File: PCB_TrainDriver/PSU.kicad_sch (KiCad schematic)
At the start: 20 parts, among them U8 TPSM863257RDXR, U9 LDL1117S33R

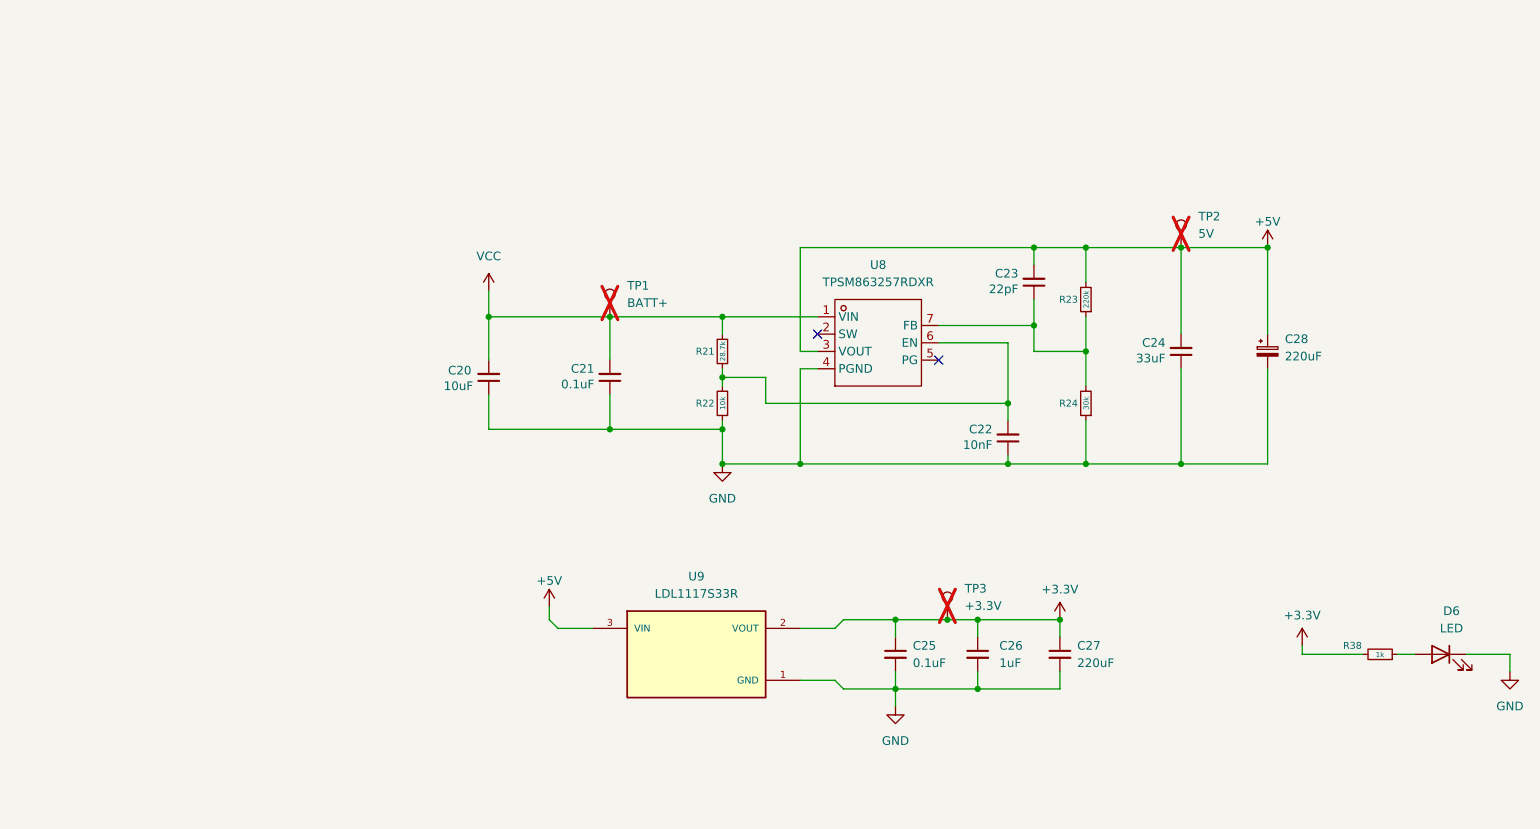
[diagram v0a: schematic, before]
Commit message: Finished sch
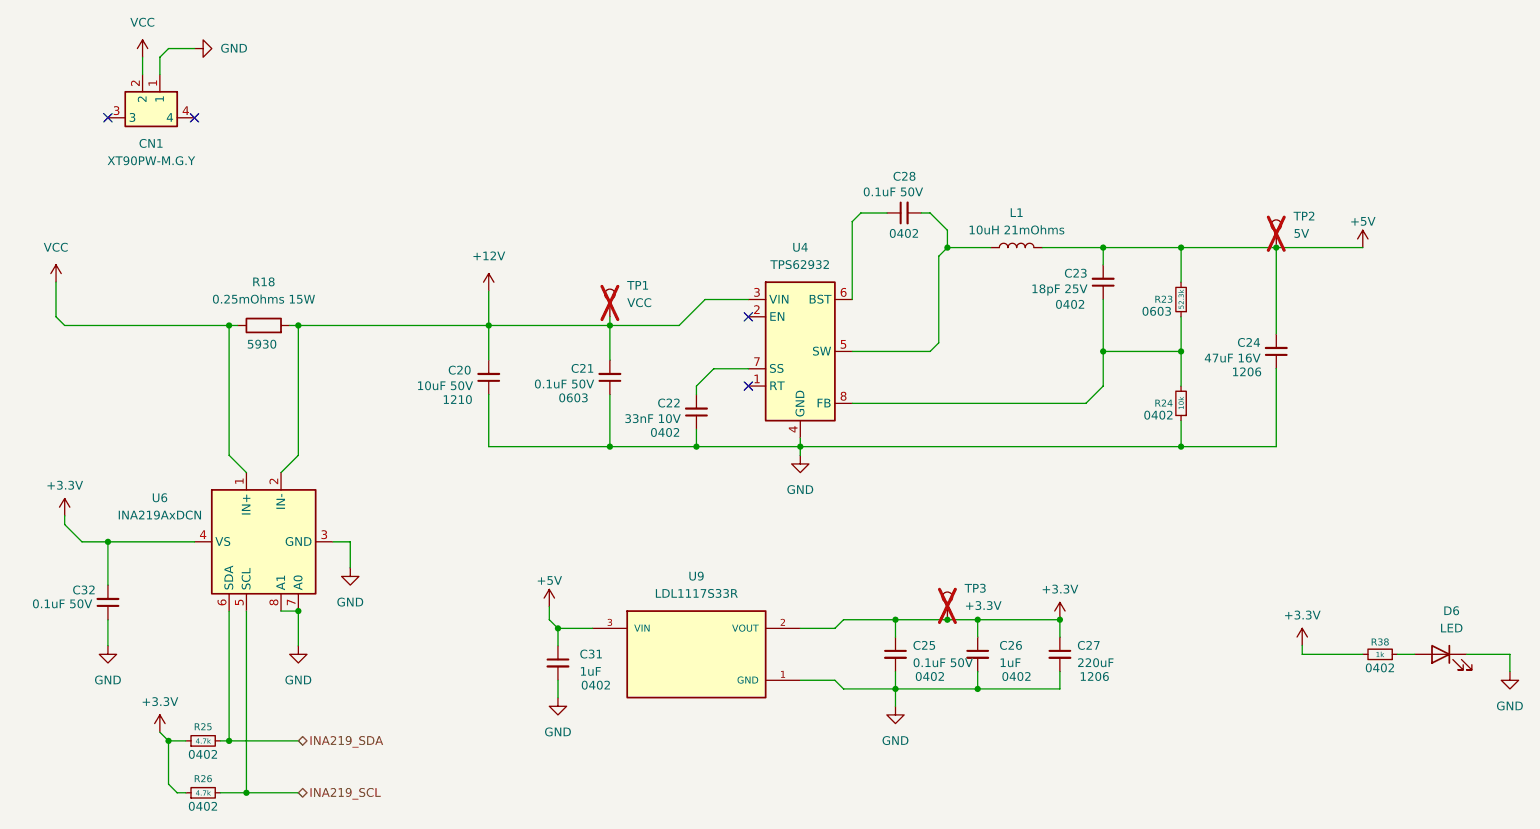
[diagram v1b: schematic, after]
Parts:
- removed C28: 220uF, Capacitor_SMD:CP_Elec_6.3x5.4, symbol Device:C_Polarized_Small
- removed R21: 28.7k, Resistor_SMD:R_0402_1005Metric, symbol Device:R_Small
- removed R22: 10k, Resistor_SMD:R_0402_1005Metric, symbol Device:R_Small
- removed U8: TPSM863257RDXR, SamacSys_Parts:QFN-7_L4.0-W3.3_TPSM863257RDXR, symbol SamacSys_Parts:TPSM863257RDXR
- added C28, C32: 0.1uF 50V, Capacitor_SMD:C_0402_1005Metric, symbol Device:C_Small
- added C31: 1uF, Capacitor_SMD:C_0402_1005Metric, symbol Device:C_Small
- added CN1: XT90PW-M.G.Y, Sharing_Footprint:CONN-TH_XT90PW-M.G.Y, symbol Sharing_Symbol:XT90PW-M.G.Y
- added L1: 10uH 21mOhms, Inductor_SMD:L_12x12mm_H4.5mm, symbol Device:L
- added R18: 0.25mOhms 15W, Sharing_Footprint:R5930, symbol Device:R
- added R25, R26: 4.7k, Resistor_SMD:R_0402_1005Metric, symbol Device:R_Small
- added U4: TPS62932, Package_TO_SOT_SMD:SOT-583-8, symbol Regulator_Switching:TPS62932
- added U6: INA219AxDCN, Package_TO_SOT_SMD:SOT-23-8, symbol Sensor_Energy:INA219AxDCN
- C20: value 10uF -> 10uF 50V; footprint Capacitor_SMD:C_0402_1005Metric -> Capacitor_SMD:C_1206_3216Metric; JLCPCB Part # (none) -> C13585; LCSC Part # C77000 -> (none); Package (none) -> 1210
- C21: value 0.1uF -> 0.1uF 50V; footprint Capacitor_SMD:C_0402_1005Metric -> Capacitor_SMD:C_0603_1608Metric; JLCPCB Part # (none) -> C14663; LCSC Part # C71687 -> (none); Package (none) -> 0603
- C22: value 10nF -> 33nF 10V; JLCPCB Part # (none) -> C527022; LCSC Part # C541371 -> (none); Package (none) -> 0402
- C23: value 22pF -> 18pF 25V; JLCPCB Part # (none) -> C526984; LCSC Part # C1555 -> (none); Package (none) -> 0402
- C24: value 33uF -> 47uF 16V; footprint Capacitor_SMD:C_0402_1005Metric -> Capacitor_SMD:C_1206_3216Metric; JLCPCB Part # (none) -> C7472975; LCSC Part # C1160 -> (none); Package (none) -> 1206
- C25: value 0.1uF -> 0.1uF 50V; JLCPCB Part # (none) -> C307331; LCSC Part # C71687 -> (none); LCSC Part# C1525 -> (none); Package (none) -> 0402
- C26: JLCPCB Part # (none) -> C52923; LCSC Part # C14445 -> (none); LCSC Part# C29266 -> (none); Package (none) -> 0402
- C27: JLCPCB Part # (none) -> C412252; LCSC Part # C412252 -> (none); LCSC Part# C412252 -> (none); Package (none) -> 1206
- D6: footprint LED_SMD:LED_0402_1005Metric -> LED_SMD:LED_0603_1608Metric; JLCPCB Part # (none) -> C2286; LCSC Part # C71911 -> (none)
- R23: value 220k -> 52.3k; footprint Resistor_SMD:R_0402_1005Metric -> Resistor_SMD:R_0603_1608Metric; JLCPCB Part # (none) -> C23198; LCSC Part # C25767 -> (none); Package (none) -> 0603
- R24: value 30k -> 10k; JLCPCB Part # (none) -> C25744; LCSC Part # C25553 -> (none); Package (none) -> 0402
- R38: JLCPCB Part # (none) -> C11702; LCSC Part # C106235 -> (none); Package (none) -> 0402
- TP1: value BATT+ -> VCC
- U9: JLCPCB Part # (none) -> C18906017; LCSC Part # C435835 -> (none); LCSC Part# C435835 -> (none)
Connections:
- net +3.3V: now also C32.2, R25.1, R26.1, U6.4 (VS)
- net +5V: now also C31.1, L1.2
- net GND: now also C31.2, C32.1, CN1.1, U4.4 (GND), U6.3 (GND), U6.7 (A0), U6.8 (A1)
- net VCC: now also CN1.2, R18.1, U6.1 (IN+); no longer C20.2, C21.2, TP1.1
- net at C22.2: now also U4.7 (SS)
- net at C23.1, R23.1, R24.2: now also U4.8 (FB)
- new net: C28.2, L1.1, U4.5 (SW)
- new net: C28.1, U4.6 (BST)
- new net +12V: C20.2, C21.2, R18.2, TP1.1, U4.3 (VIN), U6.2 (IN-)
- new net INA219_SCL: R26.2, U6.5 (SCL)
- new net INA219_SDA: R25.2, U6.6 (SDA)
- no-connect marks 2 -> 4
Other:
- moved on the sheet: C22, C23, C24, R23, R24, TP2

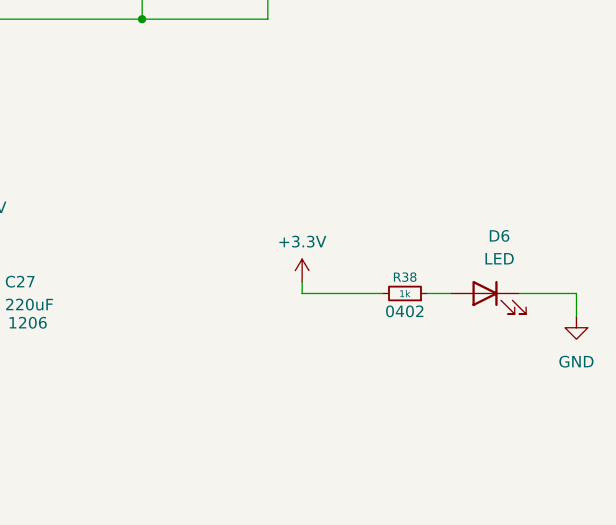
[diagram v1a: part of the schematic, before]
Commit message: PCB Almost Finished
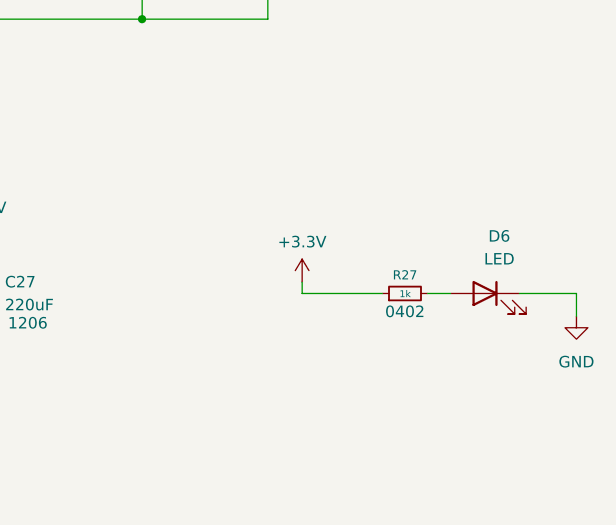
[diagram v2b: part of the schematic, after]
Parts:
- removed R38: 1k, Resistor_SMD:R_0402_1005Metric, symbol Device:R_Small
- added R27: 1k, Resistor_SMD:R_0402_1005Metric, symbol Device:R_Small
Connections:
- net +3.3V: now also R27.1
- net at D6.2 (A): now also R27.2
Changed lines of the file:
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@@
-	)
-	(symbol
-		(lib_id "Device:R_Small")
-		(at 218.44 142.24 270)
-		(mirror x)
-		(unit 1)
-		(body_style 1)
-		(exclude_from_sim no)
-		(in_bom yes)
-		(on_board no)
-		(in_pos_files yes)
-		(dnp no)
-		(property "Reference" "R38"
-			(at 218.44 140.462 90)
-			(show_name no)
-			(do_not_autoplace no)
-			(effects
-				(font
-					(size 1.016 1.016)
-				)
-			)
-		)
-		(property "Value" "1k"
-			(at 218.421 142.2933 90)
-			(show_name no)
-			(do_not_autoplace no)
-			(effects
-				(font
-					(size 0.762 0.762)
-				)
-			)
-		)
-		(property "Footprint" "Resistor_SMD:R_0402_1005Metric"
-			(at 218.44 142.24 0)
-			(hide yes)
-			(show_name no)
-			(do_not_autoplace no)
-			(effects
-				(font
-					(size 1.27 1.27)
-				)
-			)
-		)
-		(property "Datasheet" ""
-			(at 218.44 142.24 0)
-			(hide yes)
-			(show_name no)
-			(do_not_autoplace no)
-			(effects
-				(font
-					(size 1.27 1.27)
-				)
-			)
-		)
-		(property "Description" "Resistor, small symbol"
-			(at 218.44 142.24 0)
-			(hide yes)
-			(show_name no)
-			(do_not_autoplace no)
-			(effects
-				(font
-					(size 1.27 1.27)
-				)
-			)
-		)
-		(property "JLCPCB Part #" "C11702"
-			(at 218.44 142.24 90)
-			(hide yes)
-			(show_name no)
-			(do_not_autoplace no)
-			(effects
-				(font
-					(size 1.27 1.27)
-				)
-			)
-		)
-		(property "Package" "0402"
-			(at 218.44 144.272 90)
-			(show_name no)
-			(do_not_autoplace no)
-			(effects
-				(font
-					(size 1.27 1.27)
-				)
-			)
-		)
-		(property "LCSC Part #" ""
-			(at 218.44 142.24 90)
-			(hide yes)
-			(show_name no)
-			(do_not_autoplace no)
-			(effects
-				(font
-					(size 1.27 1.27)
-				)
-			)
-		)
-		(property "LCSC Part#" ""
-			(at 218.44 142.24 90)
-			(hide yes)
-			(show_name no)
-			(do_not_autoplace no)
-			(effects
-				(font
-					(size 1.27 1.27)
-				)
-			)
-		)
-		(pin "1"
-		)
-		(pin "2"
-		)
-		(instances
-			(project "PCB_TrainDriver"
-				(path "/f74253cb-ef08-441b-b3c3-36bc664bf8d8/4e4ac9ff-7b76-4f1d-9093-ce2b1ba9f40d"
-					(reference "R38")
-					(unit 1)
-				)
-			)
-		)
 	)
 	(symbol
@@
 					(unit 1)
 				)
+			)
+		)
+	)
+	(symbol
+		(lib_id "Device:R_Small")
+		(at 218.44 142.24 90)
+		(unit 1)
+		(body_style 1)
+		(exclude_from_sim no)
+		(in_bom yes)
+		(on_board yes)
+		(in_pos_files yes)
+		(dnp no)
+		(property "Reference" "R27"
+			(at 218.44 140.208 90)
+			(show_name no)
+			(do_not_autoplace no)
+			(effects
+				(font
+					(size 1.016 1.016)
+				)
+			)
+		)
+		(property "Value" "1k"
+			(at 218.459 142.2933 90)
+			(show_name no)
+			(do_not_autoplace no)
+			(effects
+				(font
+					(size 0.762 0.762)
+				)
+			)
+		)
+		(property "Footprint" "Resistor_SMD:R_0402_1005Metric"
+			(at 218.44 142.24 0)
+			(hide yes)
+			(show_name no)
+			(do_not_autoplace no)
+			(effects
+				(font
+					(size 1.27 1.27)
+				)
+			)
+		)
+		(property "Datasheet" ""
+			(at 218.44 142.24 0)
+			(hide yes)
+			(show_name no)
+			(do_not_autoplace no)
+			(effects
+				(font
+					(size 1.27 1.27)
+				)
+			)
+		)
+		(property "Description" "Resistor, small symbol"
+			(at 218.44 142.24 0)
+			(hide yes)
+			(show_name no)
+			(do_not_autoplace no)
+			(effects
+				(font
+					(size 1.27 1.27)
+				)
+			)
+		)
+		(property "JLCPCB Part #" "C25900"
+			(at 218.44 142.24 0)
+			(hide yes)
+			(show_name no)
+			(do_not_autoplace no)
+			(effects
+				(font
+					(size 1.27 1.27)
+				)
+			)
+		)
+		(property "Package" "0402"
+			(at 218.44 144.272 90)
+			(show_name no)
+			(do_not_autoplace no)
+			(effects
+				(font
+					(size 1.27 1.27)
+				)
+			)
+		)
+		(property "LCSC Part #" ""
+			(at 218.44 142.24 90)
+			(hide yes)
+			(show_name no)
+			(do_not_autoplace no)
+			(effects
+				(font
+					(size 1.27 1.27)
+				)
+			)
+		)
+		(property "LCSC Part#" ""
+			(at 218.44 142.24 90)
+			(hide yes)
+			(show_name no)
+			(do_not_autoplace no)
+			(effects
+				(font
+					(size 1.27 1.27)
+				)
+			)
+		)
+		(pin "1"
+		)
+		(pin "2"
+		)
+		(instances
+			(project "PCB_TrainDriver"
+				(path "/f74253cb-ef08-441b-b3c3-36bc664bf8d8/4e4ac9ff-7b76-4f1d-9093-ce2b1ba9f40d"
+					(reference "R27")
+					(unit 1)
+				)
